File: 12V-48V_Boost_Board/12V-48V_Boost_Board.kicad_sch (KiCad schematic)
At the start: 3 parts

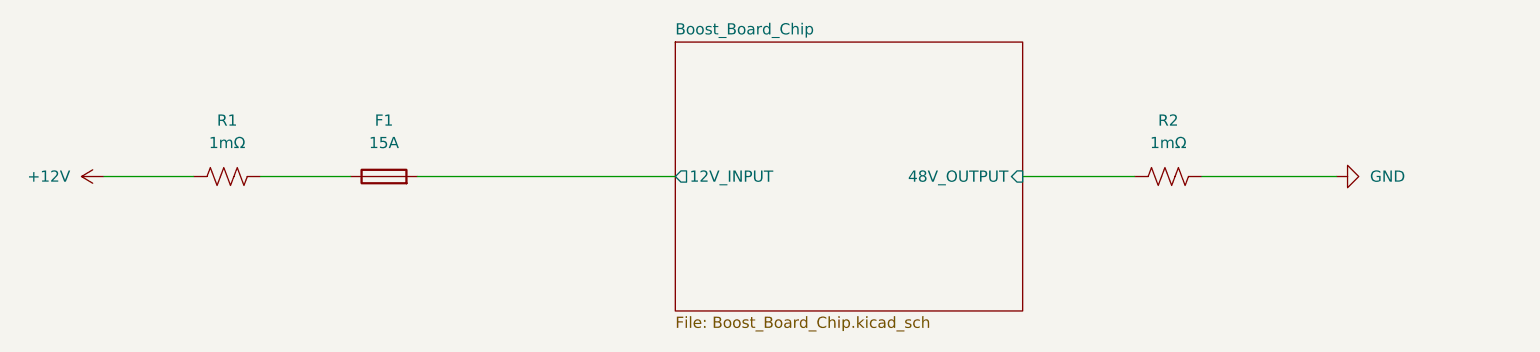
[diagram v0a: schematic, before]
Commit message: Implemented feedback from request
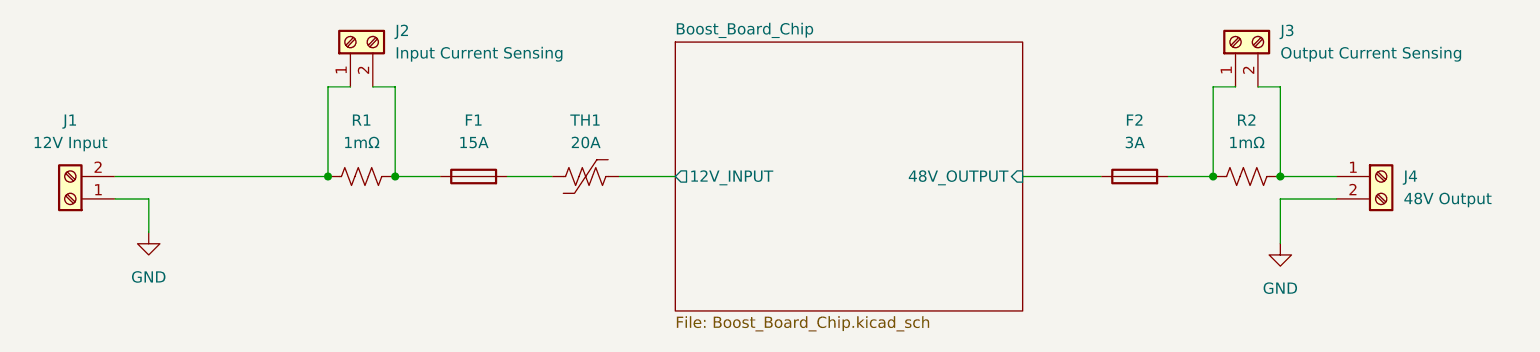
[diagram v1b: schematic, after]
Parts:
- added F2: 3A, Fuse:Fuse_0805_2012Metric_Pad1.15x1.40mm_HandSolder, symbol Device:Fuse
- added J1: 12V Input, TerminalBlock_Phoenix:TerminalBlock_Phoenix_PT-1,5-2-5.0-H_1x02_P5.00mm_Horizontal, symbol Connector:Screw_Terminal_01x02
- added J2: Input Current Sensing, TerminalBlock_Phoenix:TerminalBlock_Phoenix_PT-1,5-2-5.0-H_1x02_P5.00mm_Horizontal, symbol Connector:Screw_Terminal_01x02
- added J3: Output Current Sensing, TerminalBlock_Phoenix:TerminalBlock_Phoenix_PT-1,5-2-5.0-H_1x02_P5.00mm_Horizontal, symbol Connector:Screw_Terminal_01x02
- added J4: 48V Output, TerminalBlock_Phoenix:TerminalBlock_Phoenix_PT-1,5-2-5.0-H_1x02_P5.00mm_Horizontal, symbol Connector:Screw_Terminal_01x02
- added TH1: 20A, symbol Device:Thermistor_US
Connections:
- net Boost_Board_Chip/12V_INPUT: now also TH1.2; no longer F1.2
- net Boost_Board_Chip/48V_OUTPUT: now also F2.1; no longer R2.1
- net GND: now also J1.1 (Pin_1), J4.2 (Pin_2); no longer R2.2
- net at F1.1, R1.2: now also J2.2 (Pin_2)
- net +12V: no longer names the net of R1.1
- net +12V: now also J1.2 (Pin_2), J2.1 (Pin_1)
- new net: J3.2 (Pin_2), J4.1 (Pin_1), R2.2
- new net: F1.2, TH1.1
- new net: F2.2, J3.1 (Pin_1), R2.1
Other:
- moved on the sheet: F1, R1, R2
